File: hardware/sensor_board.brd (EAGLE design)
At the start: 50 x 17 mm, 11 parts, among them X5 i2c

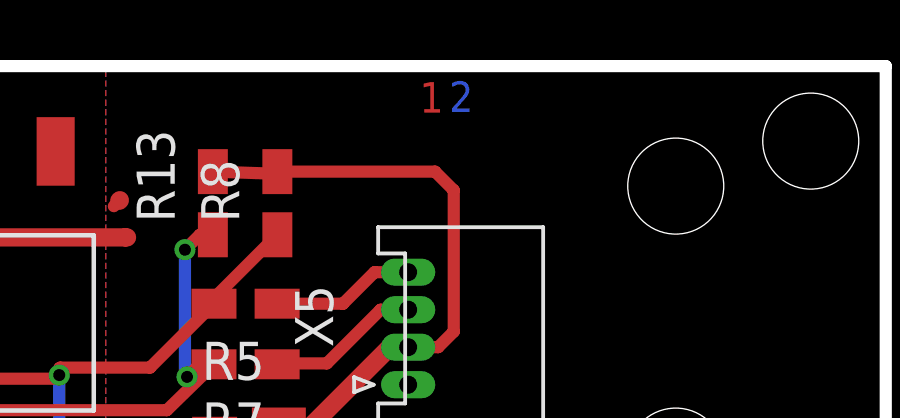
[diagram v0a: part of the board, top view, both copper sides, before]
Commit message: board ready
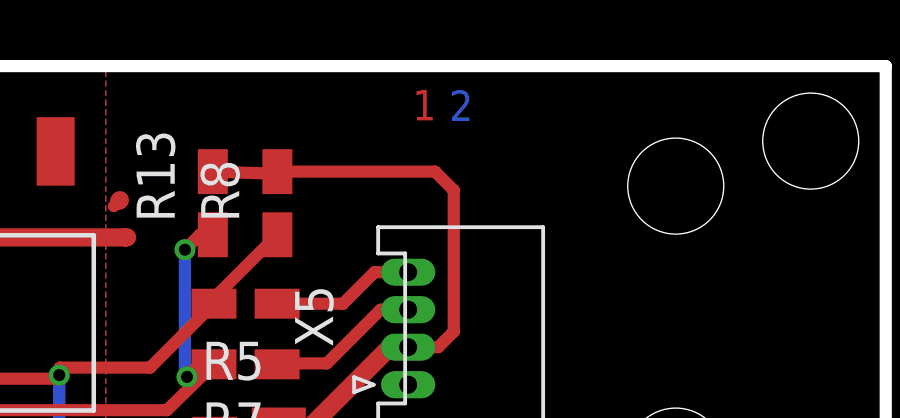
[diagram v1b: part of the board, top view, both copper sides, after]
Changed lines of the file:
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@@
 <layers>
 <layer number="1" name="Top" color="4" fill="1" visible="yes" active="yes"/>
-<layer number="2" name="Route2" color="1" fill="3" visible="yes" active="yes"/>
+<layer number="2" name="Route2" color="1" fill="3" visible="no" active="no"/>
 <layer number="3" name="Route3" color="4" fill="3" visible="no" active="no"/>
 <layer number="14" name="Route14" color="1" fill="6" visible="no" active="no"/>
-<layer number="15" name="Route15" color="4" fill="6" visible="yes" active="yes"/>
+<layer number="15" name="Route15" color="4" fill="6" visible="no" active="no"/>
 <layer number="16" name="Bottom" color="1" fill="1" visible="yes" active="yes"/>
 <layer number="17" name="Pads" color="2" fill="1" visible="yes" active="yes"/>
@@
 <hole x="47.5" y="14.5" drill="3.2"/>
 <rectangle x1="19.7" y1="6.5" x2="21.2" y2="8" layer="30"/>
-<text x="34.46" y="15.45" size="1.016" layer="1" font="vector" ratio="15">1</text>
-<text x="36.25" y="16.49" size="1.016" layer="16" font="vector" ratio="15" rot="R180">2</text>
+<text x="34.22" y="15.19" size="1.016" layer="1" font="vector" ratio="15">1</text>
+<text x="35.45" y="15.17" size="1.016" layer="16" font="vector" ratio="15">2</text>
 <wire x1="4.7" y1="41.06" x2="7.5" y2="41.06" width="1.6764" layer="42"/>
 <rectangle x1="17.8" y1="5.1" x2="21.8" y2="9.4" layer="30"/>
@@
 </class>
 </classes>
-<designrules name="SeeedStudio_DRU_no_angle_20130527">
+<designrules name="seeed_2-layer_20140221">
 <description language="de">&lt;b&gt;EAGLE Design Rules&lt;/b&gt;
 &lt;p&gt;
@@
 <description language="zh">&lt;b&gt;Seeed Studio EAGLE Design Rules&lt;/b&gt;
 </description>
-<param name="layerSetup" value="(1*2*15*16)"/>
+<param name="layerSetup" value="(1*16)"/>
 <param name="mtCopper" value="0.035mm 0.0175mm 0.035mm 0.035mm 0.035mm 0.035mm 0.035mm 0.035mm 0.035mm 0.035mm 0.035mm 0.035mm 0.035mm 0.035mm 0.0175mm 0.035mm"/>
-<param name="mtIsolate" value="0.2mm 1.1mm 0.2mm 0.15mm 0.2mm 0.15mm 0.2mm 0.15mm 0.2mm 0.15mm 0.2mm 0.15mm 0.2mm 0.15mm 0.2mm"/>
+<param name="mtIsolate" value="1.5mm 1.1mm 0.2mm 0.15mm 0.2mm 0.15mm 0.2mm 0.15mm 0.2mm 0.15mm 0.2mm 0.15mm 0.2mm 0.15mm 0.2mm"/>
 <param name="mdWireWire" value="6mil"/>
 <param name="mdWirePad" value="6mil"/>
@@
 <param name="rlMinPadTop" value="6mil"/>
 <param name="rlMaxPadTop" value="20mil"/>
-<param name="rlMinPadInner" value="6mil"/>
+<param name="rlMinPadInner" value="10mil"/>
 <param name="rlMaxPadInner" value="20mil"/>
 <param name="rlMinPadBottom" value="6mil"/>
@@
 <param name="mlMinCreamFrame" value="0mil"/>
 <param name="mlMaxCreamFrame" value="0mil"/>
-<param name="mlViaStopLimit" value="25mil"/>
+<param name="mlViaStopLimit" value="100mil"/>
 <param name="srRoundness" value="0"/>
 <param name="srMinRoundness" value="0mil"/>
